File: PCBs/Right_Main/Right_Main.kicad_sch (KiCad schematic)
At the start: 13 parts, among them J10 Rotary switch pins 1, J5 Conn_IDC_Right_To_Left, J6 Screw terminal 5V GND Out, J7 Encoder inputs B, J8 Encoder inputs A, J9 Analog Inputs, U5 MCP23017_SP, U6 74HC4051, U7 ULN2003A

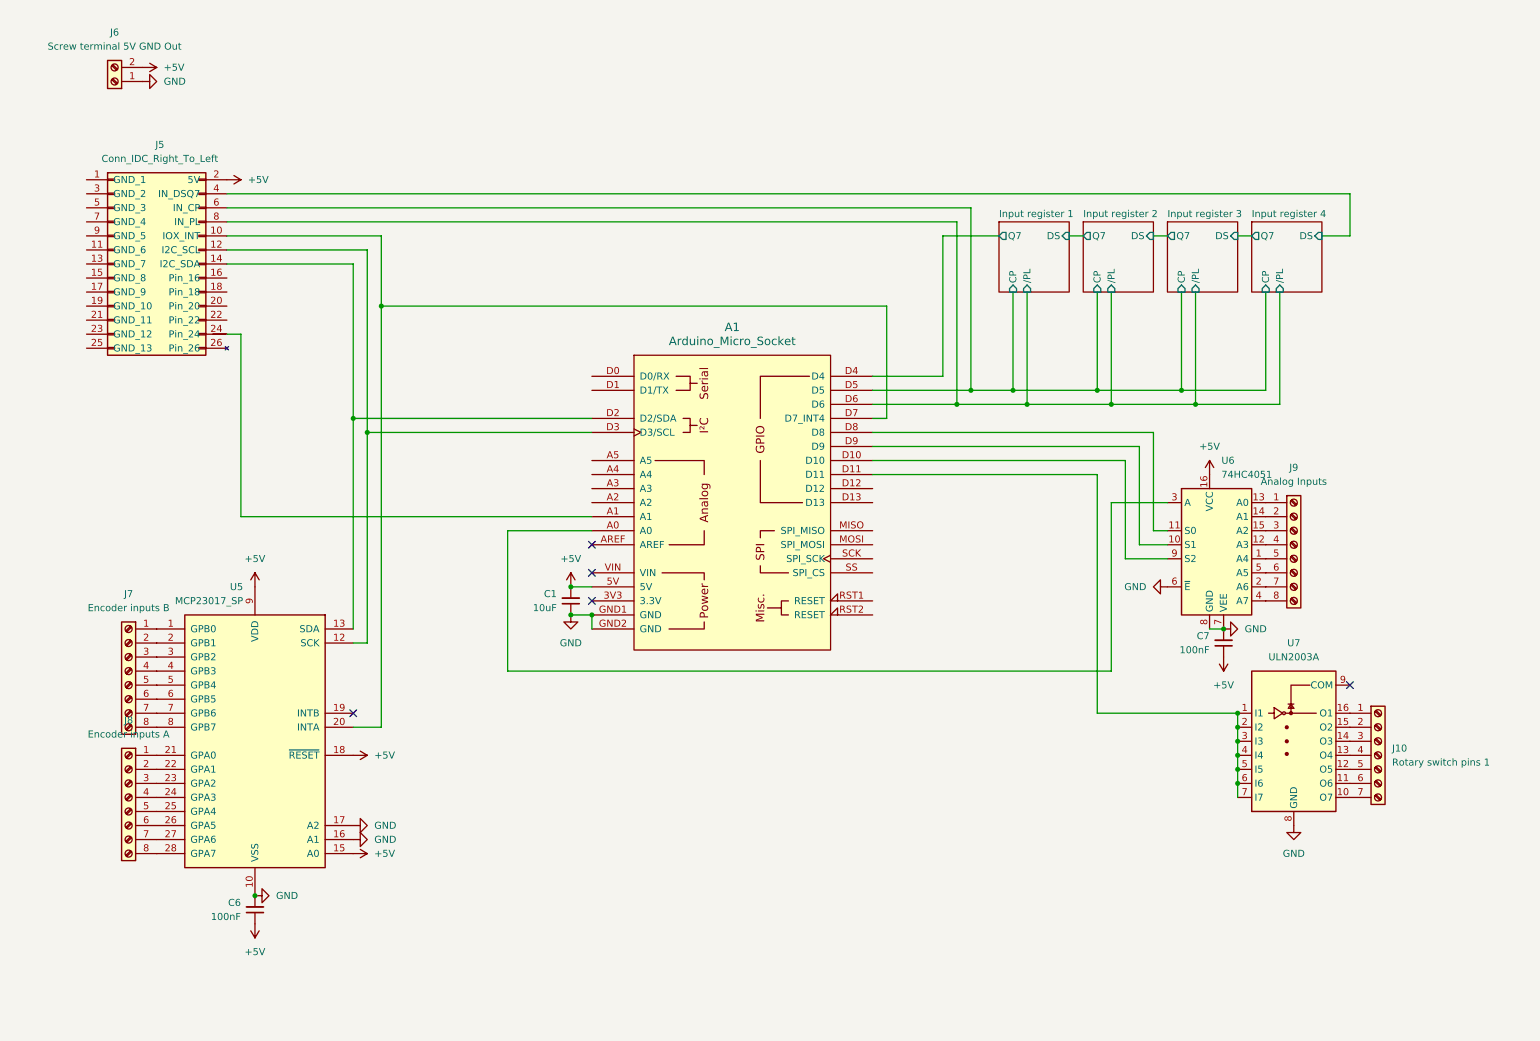
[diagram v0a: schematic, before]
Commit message: wip
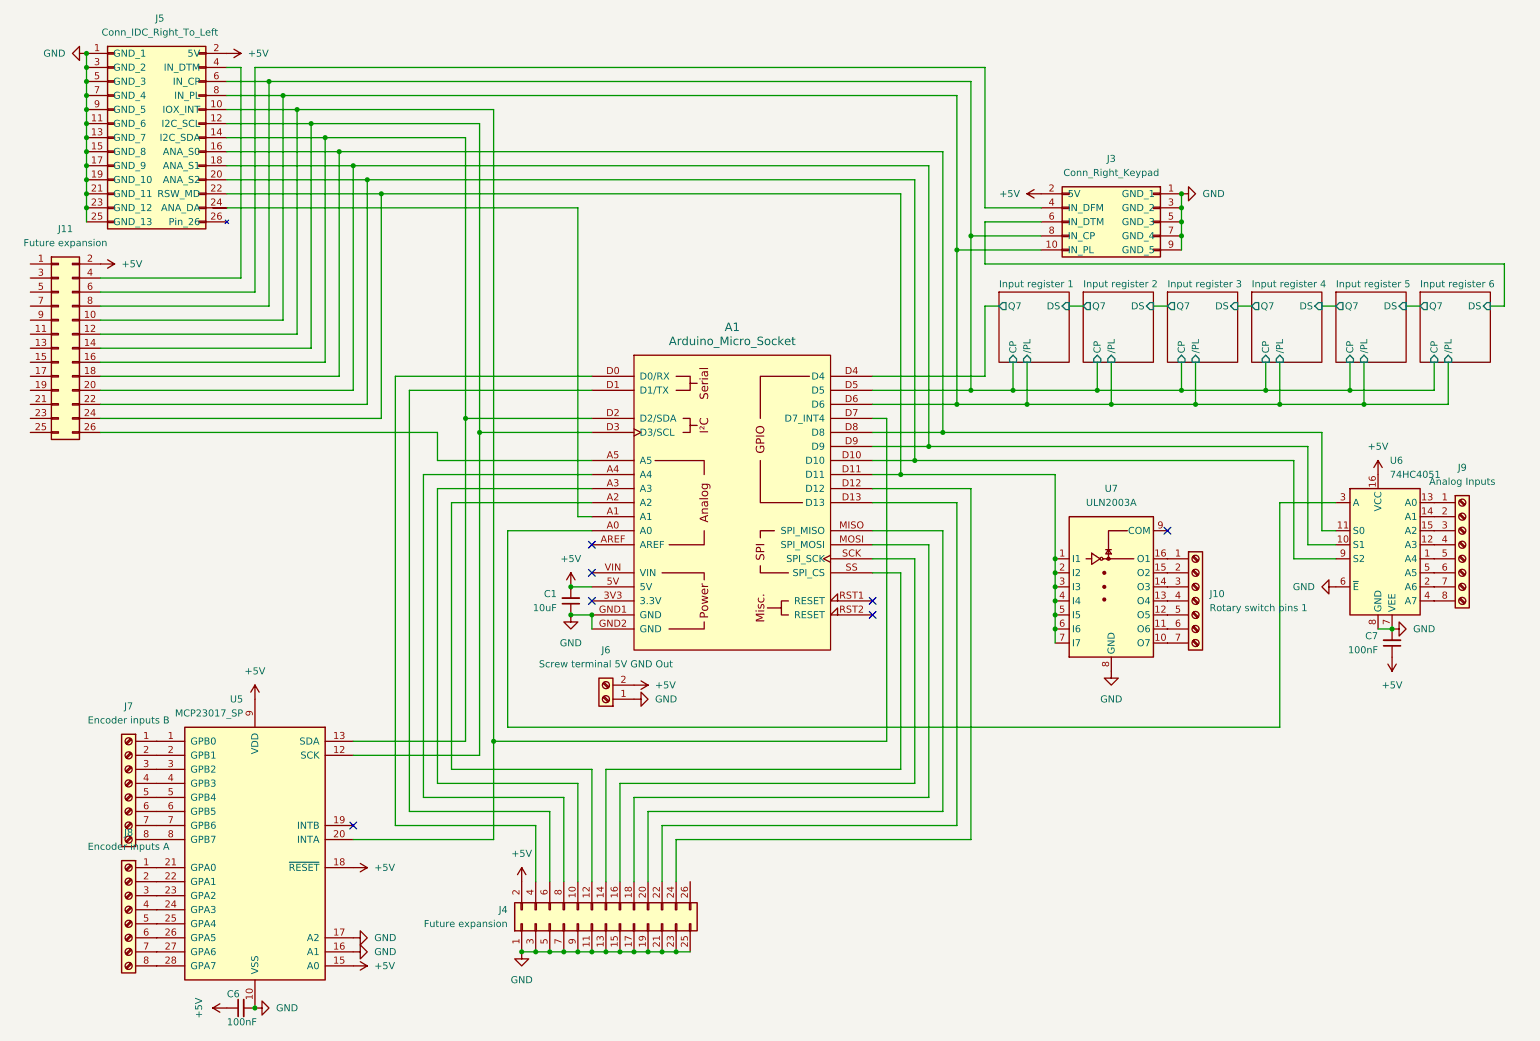
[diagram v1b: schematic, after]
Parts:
- added J11, J4: Future expansion, symbol Connector_Generic:Conn_02x13_Odd_Even
- added J3: Conn_Right_Keypad, symbol System_Connectors:Conn_Right_Keypad
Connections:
- net +5V: now also J11.2 (Pin_2), J3.2 (5V), J4.2 (Pin_2)
- net GND: now also J5.1 (GND_1), J5.11 (GND_6), J5.13 (GND_7), J5.15 (GND_8), J5.17 (GND_9), J5.19 (GND_10), J5.21 (GND_11), J5.23 (GND_12), J5.25 (GND_13), J5.3 (GND_2), J5.5 (GND_3), J5.7 (GND_4), J5.9 (GND_5), J3.1 (GND_1), J3.3 (GND_2), J3.5 (GND_3), J3.7 (GND_4), J3.9 (GND_5), J4.1 (Pin_1), J4.11 (Pin_11), J4.13 (Pin_13), J4.15 (Pin_15), J4.17 (Pin_17), J4.19 (Pin_19), J4.21 (Pin_21), J4.23 (Pin_23), J4.25 (Pin_25), J4.3 (Pin_3), J4.5 (Pin_5), J4.7 (Pin_7), J4.9 (Pin_9)
- net Input register 1/CP: now also J11.8 (Pin_8), J3.8 (IN_CP)
- net Input register 1//PL: now also J11.10 (Pin_10), J3.10 (IN_PL)
- net Input register 4/DS: no longer J5.4 (IN_DSQ7)
- net at A1.D9, U6.10 (S1): now also J5.18 (ANA_S1), J11.20 (Pin_20)
- net at A1.D8, U6.11 (S0): now also J5.16 (ANA_S0), J11.18 (Pin_18)
- net at A1.D10, U6.9 (S2): now also J5.20 (ANA_S2), J11.22 (Pin_22)
- net at A1.A2: now also J4.12 (Pin_12)
- net at A1.A3: now also J4.10 (Pin_10)
- net at A1.A4: now also J4.8 (Pin_8)
- net at A1.A5: now also J11.26 (Pin_26)
- net at A1.D0 (D0/RX): now also J4.4 (Pin_4)
- net at A1.D1 (D1/TX): now also J4.6 (Pin_6)
- net at A1.D11, U7.1 (I1), U7.2 (I2)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: now also J5.22 (RSW_MD), J11.24 (Pin_24)
- net at A1.D12: now also J4.24 (Pin_24)
- net at A1.D13: now also J4.22 (Pin_22)
- net at A1.D2 (D2/SDA), J5.14 (I2C_SDA), U5.13 (SDA): now also J11.16 (Pin_16)
- net at A1.D3 (D3/SCL), J5.12 (I2C_SCL), U5.12 (SCK): now also J11.14 (Pin_14)
- net at A1.D7 (D7_INT4), J5.10 (IOX_INT), U5.20 (INTA): now also J11.12 (Pin_12)
- net at A1.MISO (SPI_MISO): now also J4.20 (Pin_20)
- net at A1.MOSI (SPI_MOSI): now also J4.18 (Pin_18)
- net at A1.SCK (SPI_SCK): now also J4.16 (Pin_16)
- net at A1.SS (SPI_CS): now also J4.14 (Pin_14)
- new net: J11.6 (Pin_6), J3.4 (IN_DFM)
- new net: J11.4 (Pin_4), J5.4 (IN_DTM)
- new net Input register 6/DS: J3.6 (IN_DTM)
- no-connect marks 5 -> 7
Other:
- added sheet Input register 5 (Input_Shift_Register.kicad_sch)
- added sheet Input register 6 (Input_Shift_Register.kicad_sch)
- moved on the sheet: C6, C7, J10, J5, J6, J7, J8, J9, U5, U6, U7
